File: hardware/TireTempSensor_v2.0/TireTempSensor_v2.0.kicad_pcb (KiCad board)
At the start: 4 copper layers, 27 x 53.8 mm, 54 parts, among them IC1 MAX15462AATA+, IC2 MLX90621ESF-BAB-000-SP, J1 SWD_01x06, J2 CAN_01x04, Q1 FQT3P20TF, SW1 RESET, U1 STM32L4P5RET6, U2 MIC5306-2.6YD5-TR, U3 SN65HVD232, Y1 16MGHz

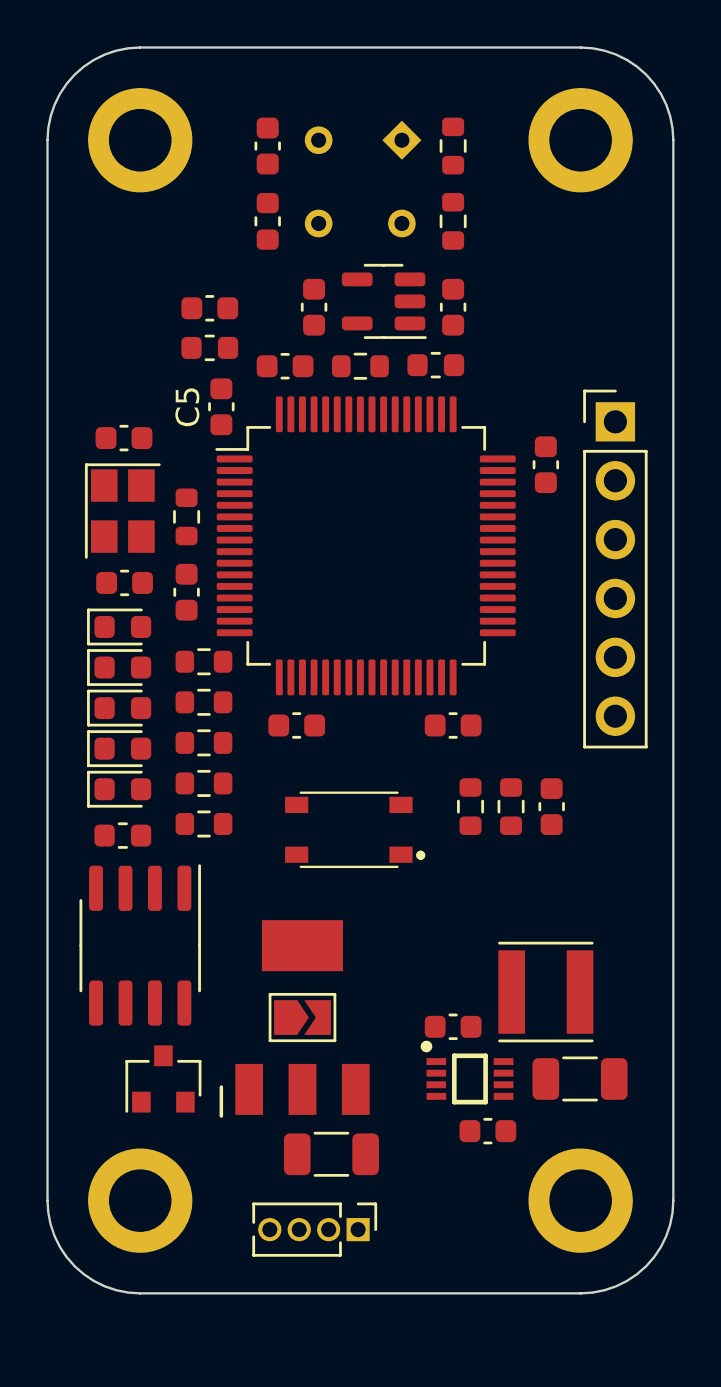
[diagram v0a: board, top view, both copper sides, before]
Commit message: some pcb connections
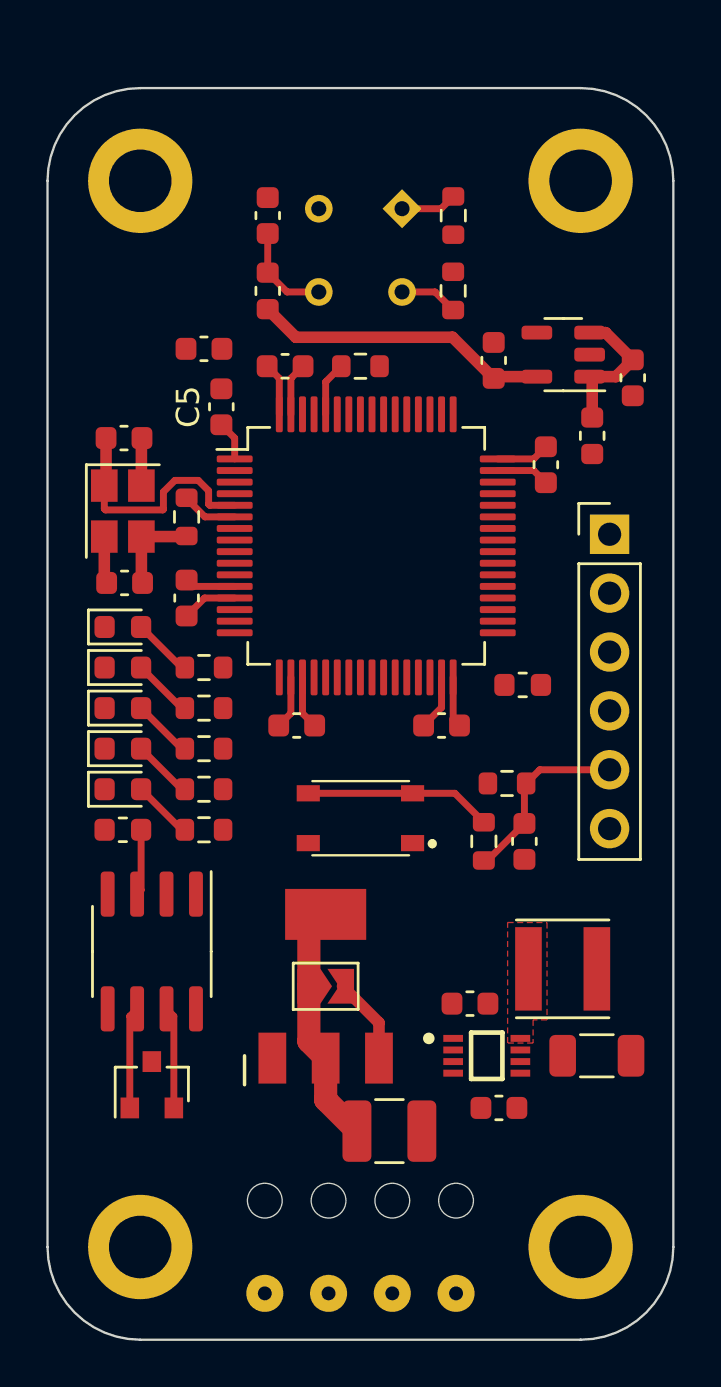
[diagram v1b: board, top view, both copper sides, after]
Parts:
- F1: footprint Capacitor_SMD:C_1206_3216Metric -> Fuse:Fuse_1210_3225Metric
- J2: footprint Connector_PinHeader_1.27mm:PinHeader_1x04_P1.27mm_Vertical -> Connector_Wire:SolderWire-0.1sqmm_1x04_P3.6mm_D0.4mm_OD1mm_Relief
- moved FB1 19.8 mm to (119.8, 89.2)
- moved C14 8.33 mm to (124.5, 76.0), turned to -90 degrees
- moved C15 8.08 mm to (118.5, 75.2)
- moved U2 8.08 mm to (121.5, 75.0)
- moved FB2 7.41 mm to (122.8, 78.5), turned to 90 degrees
- moved J2 5.04 mm to (116.9, 115.5), turned to 180 degrees
- moved J1 4.86 mm to (123.5, 82.8)
- moved R6 3.00 mm to (116.8, 69.0)
- moved C17 3.00 mm to (108.8, 69.0)
- moved FB3 3.00 mm to (108.8, 72.2)
- moved R5 3.00 mm to (116.8, 72.2)
- moved IC2 2.95 mm to (114.5, 68.7)
- moved F1 2.69 mm to (114.0, 108.5)
- moved H1 2.00 mm to (122.2, 113.5)
- moved H2 2.00 mm to (103.2, 113.5)
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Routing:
- net GND: track 0.00 -> 15.6 mm
- net /+3V3_uC: track 0.00 -> 13.2 mm
- net +2V6: track 0.00 -> 12.9 mm
- net /OSC IN: track 0.00 -> 10.6 mm
- net Net-(F1-Pad2): track 0.00 -> 10.5 mm
- net Net-(R3-Pad1): track 0.00 -> 8.09 mm
- net /NRST: track 0.00 -> 8.01 mm
- net Net-(C14-Pad1): track 0.00 -> 6.32 mm
- net /CAN L: track 0.00 -> 4.41 mm
- net /CAN H: track 0.00 -> 4.41 mm
- net Net-(C17-Pad1): track 0.00 -> 4.24 mm
- net Net-(C10-Pad1): track 0.00 -> 3.98 mm
- net /Power Supply 3.3v 2.6v/+24V safe: track 0.00 -> 3.75 mm
- net Net-(FB4-Pad2): track 0.00 -> 2.85 mm
- net Net-(D6-Pad2): track 0.00 -> 2.61 mm
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- added copper zone on In1.Cu, net GND
- added copper zone on F.Cu, net Net-(L1-Pad1)
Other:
- board size 27 x 53.8 mm -> 27 x 54 mm
